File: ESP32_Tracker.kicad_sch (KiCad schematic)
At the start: 61 parts, among them J1 USB_C_Receptacle_USB2.0_16P, J2 Conn_01x02_Socket, J3 Micro_SD_Card_Det1, SW1 SW_Push, SW2 SW_Push, SW3 SW_Push, U1 XC6220B331MR-G, U2 USBLC6-2SC6, U3 MP2667, U4 SAM-M10Q, U5 LIS2MDL, U6 ESP32-S3-MINI-1

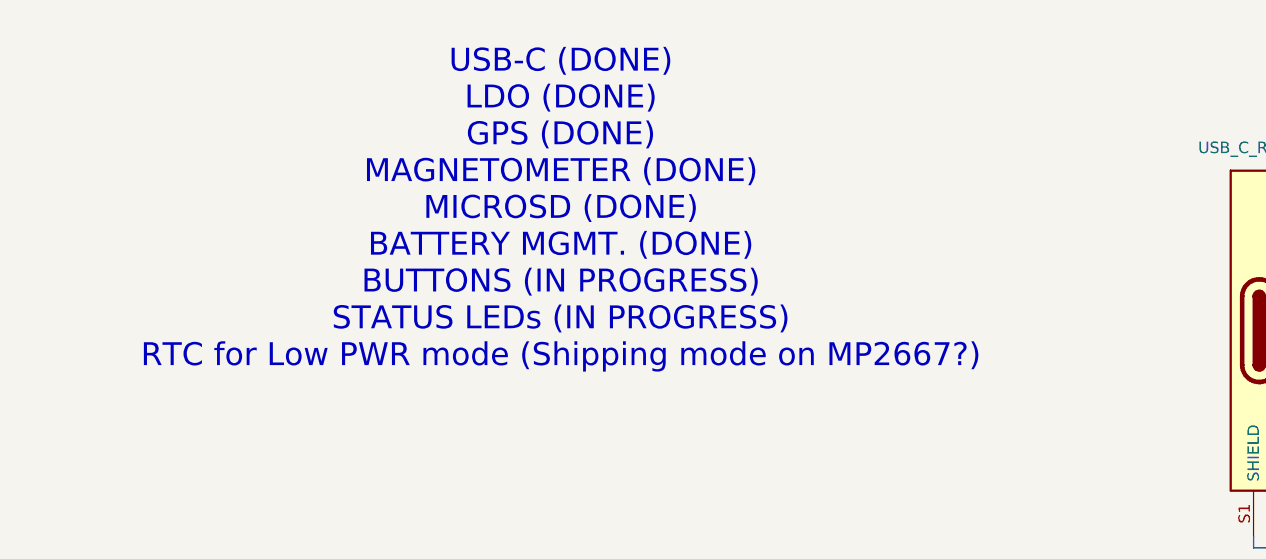
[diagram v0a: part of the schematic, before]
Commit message: models added
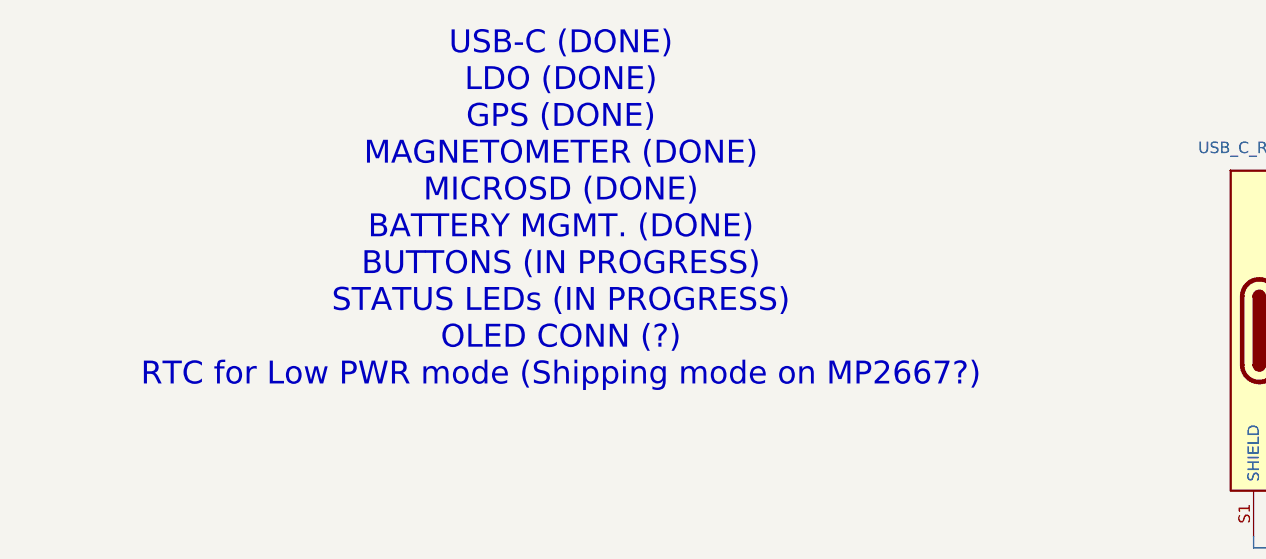
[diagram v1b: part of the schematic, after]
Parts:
- D1: footprint (none) -> LED_SMD:LED_0805_2012Metric; Distributor Link (none) -> https://www.lcsc.com/product-detail/C965812.html; LCSC (none) -> C965812; MPN (none) -> XL-2012SURC; Manufacturer (none) -> XINGLIGHT
- J3: footprint (none) -> MSD-4-A_DL:CUI_MSD-4-A; Distributor Link (none) -> https://www.digikey.com/en/products/detail/same-sky-formerl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; MPN (none) -> MSD-4-A; Manufacturer (none) -> Same Sky (Formerly CUI Devices)
- U3: footprint (none) -> MP2667_DL:QFN-10_2MMx2MM_MNP; Distributor Link (none) -> https://www.digikey.com/en/products/detail/monolithic-power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; MPN (none) -> MP2667GG-0000-Z; Manufacturer (none) -> Monolithic Power Systems Inc.
- U4: MPN (none) -> SAM-M10Q-00B; Manufacturer (none) -> u-blox
- U5: MPN (none) -> LIS2MDLTR; Manufacturer (none) -> STMicroelectronics
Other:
- note added: "USB-C (DONE) LDO (DONE) GPS (DONE) MAGNETOMETER (DONE) MICROSD (DONE) BATTERY MGMT. (DONE) BUTTONS (IN PROGRESS) STATUS LEDs (IN PROGRESS) OLED CONN (?) RTC for Low PWR mode (Shipping mode on MP2667?)"
- note removed: "USB-C (DONE) LDO (DONE) GPS (DONE) MAGNETOMETER (DONE) MICROSD (DONE) BATTERY MGMT. (DONE) BUTTONS (IN PROGRESS) STATUS LEDs (IN PROGRESS) RTC for Low PWR mode (Shipping mode on MP2667?)"
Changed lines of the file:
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@@
 		)
 	)
-	(text "USB-C (DONE)\nLDO (DONE)\nGPS (DONE)\nMAGNETOMETER (DONE)\nMICROSD (DONE)\nBATTERY MGMT. (DONE)\nBUTTONS (IN PROGRESS)\nSTATUS LEDs (IN PROGRESS)\nRTC for Low PWR mode (Shipping mode on MP2667?)"
+	(text "USB-C (DONE)\nLDO (DONE)\nGPS (DONE)\nMAGNETOMETER (DONE)\nMICROSD (DONE)\nBATTERY MGMT. (DONE)\nBUTTONS (IN PROGRESS)\nSTATUS LEDs (IN PROGRESS)\nOLED CONN (?)\nRTC for Low PWR mode (Shipping mode on MP2667?)"
 		(exclude_from_sim no)
 		(at -55.372 29.718 0)
@@
 			)
 		)
-		(property "MPN" ""
+		(property "MPN" "LIS2MDLTR"
 			(at 204.47 139.7 0)
 			(effects
@@
 			)
 		)
-		(property "Manufacturer" ""
+		(property "Manufacturer" "STMicroelectronics"
 			(at 204.47 139.7 0)
 			(effects
@@
 			)
 		)
-		(property "Footprint" ""
+		(property "Footprint" "MP2667_DL:QFN-10_2MMx2MM_MNP"
 			(at 148.59 43.18 0)
 			(effects
@@
 			)
 		)
+		(property "Distributor Link" "https://www.digikey.com/en/products/detail/monolithic-power-systems-inc/MP2667GG-0000-Z/11611000"
+			(at 148.59 43.18 0)
+			(effects
+				(font
+					(size 1.27 1.27)
+				)
+				(hide yes)
+			)
+		)
+		(property "MPN" "MP2667GG-0000-Z"
+			(at 148.59 43.18 0)
+			(effects
+				(font
+					(size 1.27 1.27)
+				)
+				(hide yes)
+			)
+		)
+		(property "Manufacturer" "Monolithic Power Systems Inc."
+			(at 148.59 43.18 0)
+			(effects
+				(font
+					(size 1.27 1.27)
+				)
+				(hide yes)
+			)
+		)
 		(pin "10"
 		)
@@
 			)
 		)
-		(property "MPN" ""
+		(property "MPN" "SAM-M10Q-00B"
 			(at 240.03 87.63 0)
 			(effects
@@
 			)
 		)
-		(property "Manufacturer" ""
+		(property "Manufacturer" "u-blox"
 			(at 240.03 87.63 0)
 			(effects
@@
 			)
 		)
-		(property "Footprint" ""
+		(property "Footprint" "MSD-4-A_DL:CUI_MSD-4-A"
 			(at 443.23 128.27 0)
 			(effects
@@
 			)
 		)
-		(property "MPN" ""
+		(property "MPN" "MSD-4-A"
 			(at 391.16 146.05 0)
 			(effects
@@
 			)
 		)
-		(property "Manufacturer" ""
+		(property "Manufacturer" "Same Sky (Formerly CUI Devices)"
+			(at 391.16 146.05 0)
+			(effects
+				(font
+					(size 1.27 1.27)
+				)
+				(hide yes)
+			)
+		)
+		(property "Distributor Link" "https://www.digikey.com/en/products/detail/same-sky-formerly-cui-devices/MSD-4-A/21796808"
 			(at 391.16 146.05 0)
 			(effects
@@
 			)
 		)
-		(property "Footprint" ""
+		(property "Footprint" "LED_SMD:LED_0805_2012Metric"
 			(at 118.11 170.18 0)
 			(effects
@@
 			)
 		)
-		(property "Datasheet" "~"
+		(property "Datasheet" "https://www.lcsc.com/datasheet/C965812.pdf"
 			(at 118.11 170.18 0)
 			(effects
@@
 			(at 118.11 170.18 0)
 			(effects
+				(font
+					(size 1.27 1.27)
+				)
+				(hide yes)
+			)
+		)
+		(property "Distributor Link" "https://www.lcsc.com/product-detail/C965812.html"
+			(at 118.11 170.18 0)
+			(effects
+				(font
+					(size 1.27 1.27)
+				)
+				(hide yes)
+			)
+		)
+		(property "LCSC" "C965812"
+			(at 118.11 170.18 0)
+			(effects
+				(font
+					(size 1.27 1.27)
+				)
+				(hide yes)
+			)
+		)
+		(property "MPN" "XL-2012SURC"
+			(at 118.11 170.18 0)
+			(effects
+				(font
+					(size 1.27 1.27)
+				)
+				(hide yes)
+			)
+		)
+		(property "Manufacturer" "XINGLIGHT"
+			(at 118.11 170.18 0)
+			(effects
